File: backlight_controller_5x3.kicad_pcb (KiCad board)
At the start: 2 copper layers, 121.3 x 67.3 mm, 58 parts, among them J1 DB9F_SMD, J10 M12-5-RCPT_F_SMD, J2 DB9M_SMD, J3 M12-5-RCPT_F_SMD, J4 M12-5-RCPT_F_SMD, J5 M12-5-RCPT_F_SMD, J6 M12-5-RCPT_F_SMD, J7 M12-5-RCPT_F_SMD, J8 M12-5-RCPT_F_SMD, J9 M12-5-RCPT_F_SMD, P1 MINI_FIT_JR_02X03_M_RA, U1 SN74ABT541BDWR, U10 NUD3124, U2 SN74ABT541BDWR, U3 NUD3124, U4 NUD3124, U5 NUD3124, U6 NUD3124, U7 NUD3124, U8 NUD3124, U9 NUD3124

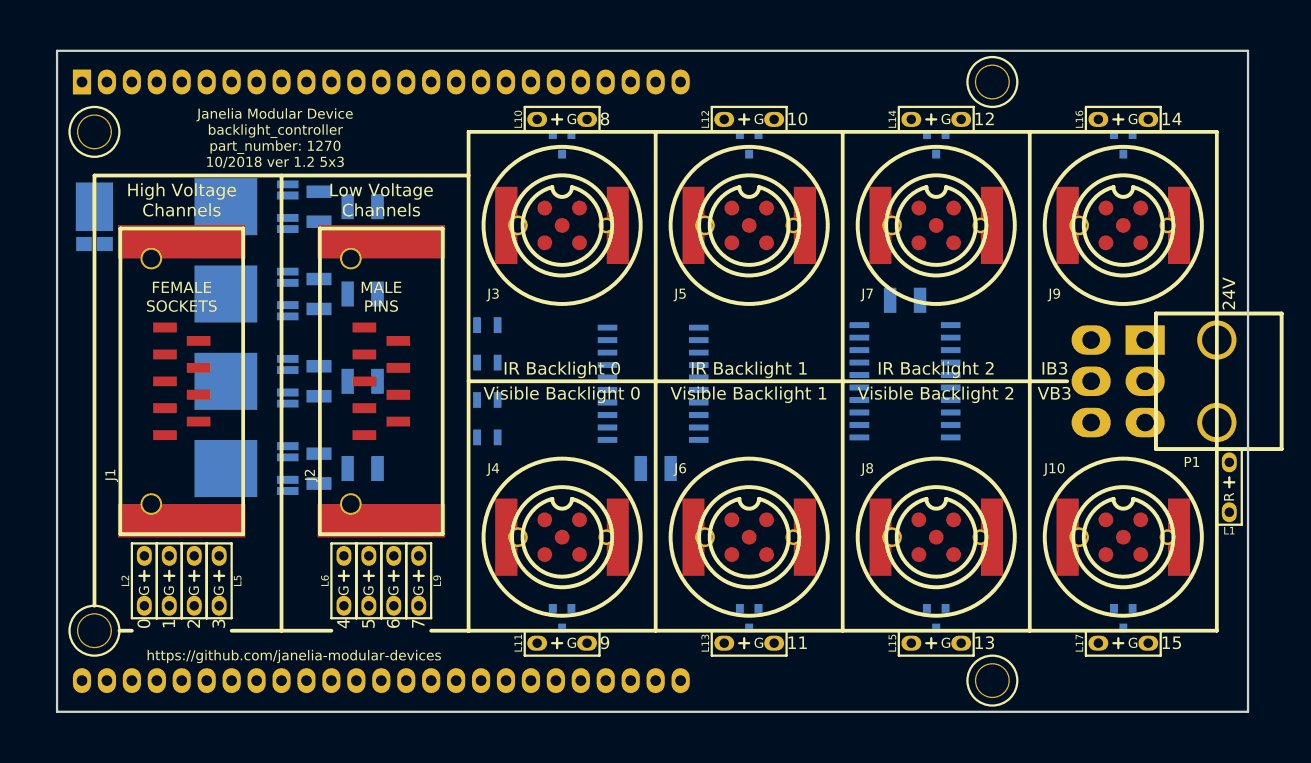
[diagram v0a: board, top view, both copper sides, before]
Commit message: Finished version 1.2.
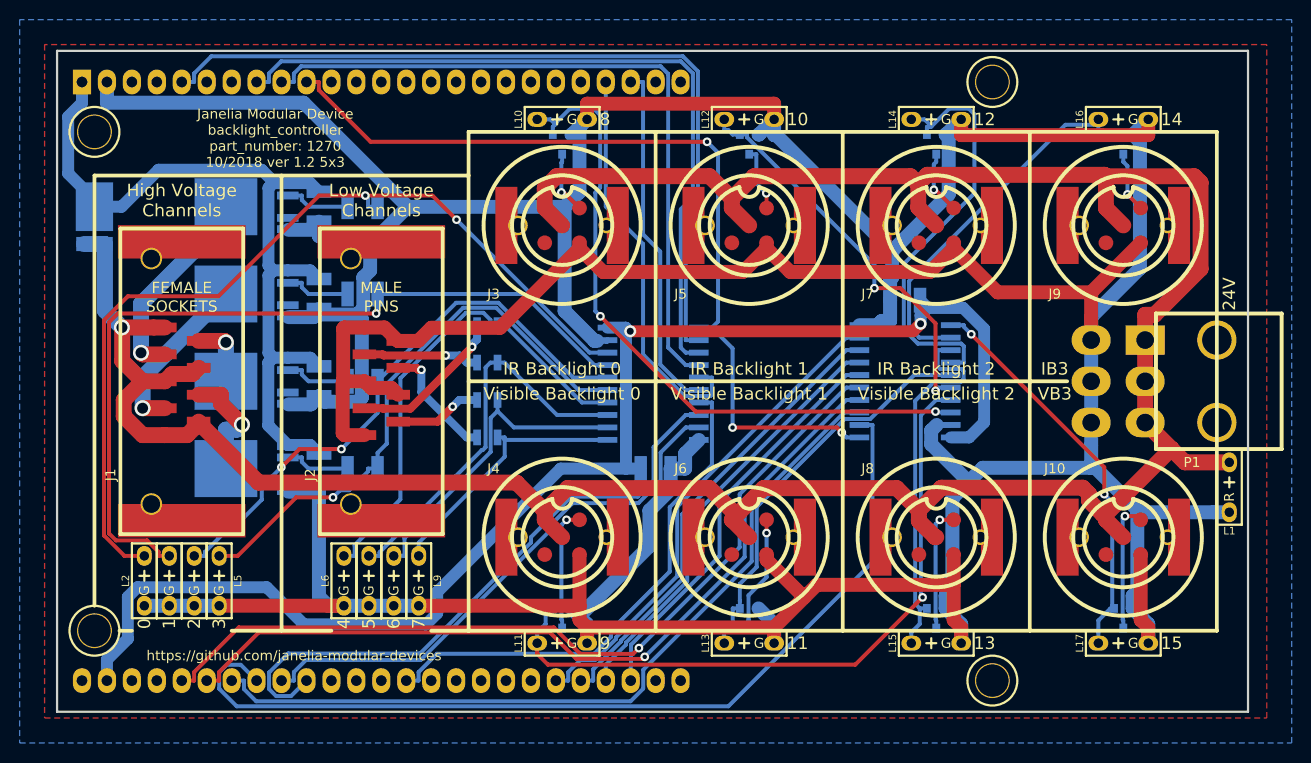
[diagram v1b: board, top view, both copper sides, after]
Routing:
- net GND: track 0.00 -> 618.1 mm
- net VAA: track 0.00 -> 293.7 mm, vias 0 -> 1
- net VEE: track 0.00 -> 141.2 mm, vias 0 -> 2
- net /CHANNEL_8: track 0.00 -> 95.1 mm
- net /backlight_5x3/C_0: track 0.00 -> 92.3 mm, vias 0 -> 2
- net /~ENABLE: track 0.00 -> 89.2 mm, vias 0 -> 3
- net /CHANNEL_11: track 0.00 -> 87.3 mm, vias 0 -> 1
- net /backlight_5x3/C_1: track 0.00 -> 84.9 mm, vias 0 -> 1
- net /CHANNEL_10: track 0.00 -> 84.3 mm, vias 0 -> 1
- net /CHANNEL_0: track 0.00 -> 84.0 mm
- net VDD: track 0.00 -> 82.7 mm
- net /CHANNEL_9: track 0.00 -> 82.0 mm
- net /CHANNEL_1: track 0.00 -> 76.8 mm
- net /CHANNEL_2: track 0.00 -> 72.6 mm
- net /backlight_5x3/C_9: track 0.00 -> 70.6 mm, vias 0 -> 1
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- added copper zone on B.Cu, net GND
- added copper zone on F.Cu, net VAA
